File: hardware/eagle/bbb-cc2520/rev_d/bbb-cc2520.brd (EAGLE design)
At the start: 54.6 x 73.4 mm, 98 parts, among them J1 TC2030-IDC, J2 JUMPER-PTH-2-NO, P9/P8 BBB_HEADERS, U1 CC2520, U2 CC2520, U3 CAT24C256WI-GT3, U4 CC2591, U5 CD4051B-53B, U6 NRF51822QF, X1 NX2520SA, X2 NX2520SA, X3 16MHz

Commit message: committing changes to gap
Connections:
- removed net A0: U6.45
- removed net A1: U6.46
- removed net CC0_GPIO0: U1.10
- removed net CC0_GPIO5: U1.4
- removed net P03: U6.7
- removed net P12: U6.18
- removed net P24: U6.43
- removed net P25: U6.44
- removed net PROG_RX: U6.47
- removed net PROG_TX: U6.48
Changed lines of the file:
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@@
 <wire x1="13.462" y1="46.482" x2="12.192" y2="45.212" width="0.2032" layer="1"/>
-</signal>
-<signal name="CC0_GPIO5">
-<contactref element="U1" pad="4"/>
-</signal>
-<signal name="CC0_GPIO0">
-<contactref element="U1" pad="10"/>
 </signal>
 <signal name="VCC">
@@
 <wire x1="26.19593125" y1="56.093" x2="25.908" y2="55.80506875" width="0.2032" layer="1"/>
 <wire x1="25.908" y1="55.80506875" x2="24.892" y2="55.80506875" width="0.2032" layer="1"/>
-<contactref element="R15" pad="2"/>
-<contactref element="R16" pad="2"/>
-<via x="23.876" y="40.132" extent="1-16" drill="0.4064"/>
-<contactref element="R14" pad="2"/>
 <wire x1="13.02893125" y1="66.04" x2="11.35506875" y2="66.04" width="0.4064" layer="1"/>
 <wire x1="11.35506875" y1="64.135" x2="11.35506875" y2="66.04" width="0.4064" layer="1"/>
@@
 <via x="24.003" y="55.626" extent="1-16" drill="0.4064"/>
 <wire x1="7.884" y1="68.448" x2="7.874" y2="68.65493125" width="0.254" layer="1"/>
+<wire x1="32.58693125" y1="19.05" x2="32.3215" y2="18.78456875" width="0.2032" layer="1"/>
+<wire x1="32.3215" y1="18.78456875" x2="32.3215" y2="17.78" width="0.2032" layer="1"/>
+<wire x1="11.35506875" y1="66.04" x2="11.35506875" y2="68.20893125" width="0.4064" layer="1"/>
+<wire x1="11.35506875" y1="68.20893125" x2="11.116" y2="68.448" width="0.4064" layer="1"/>
+<wire x1="19.812" y1="40.894" x2="19.893" y2="40.813" width="0.2032" layer="1"/>
+<wire x1="19.893" y1="40.813" x2="19.893" y2="39.867" width="0.2032" layer="1"/>
+<contactref element="R15" pad="2"/>
+<contactref element="R16" pad="2"/>
+<contactref element="R14" pad="2"/>
+<via x="23.876" y="40.132" extent="1-16" drill="0.4064"/>
 <wire x1="24.05506875" y1="37.846" x2="24.05506875" y2="38.42893125" width="0.2032" layer="1"/>
 <wire x1="24.05506875" y1="38.42893125" x2="23.368" y2="39.116" width="0.2032" layer="1"/>
 <wire x1="23.368" y1="39.116" x2="22.78506875" y2="39.116" width="0.2032" layer="1"/>
 <wire x1="22.78506875" y1="41.148" x2="23.368" y2="41.148" width="0.2032" layer="1"/>
-<wire x1="32.58693125" y1="19.05" x2="32.3215" y2="18.78456875" width="0.2032" layer="1"/>
-<wire x1="32.3215" y1="18.78456875" x2="32.3215" y2="17.78" width="0.2032" layer="1"/>
-<wire x1="11.35506875" y1="66.04" x2="11.35506875" y2="68.20893125" width="0.4064" layer="1"/>
-<wire x1="11.35506875" y1="68.20893125" x2="11.116" y2="68.448" width="0.4064" layer="1"/>
 <wire x1="23.368" y1="41.148" x2="23.876" y2="40.64" width="0.2032" layer="1"/>
 <wire x1="23.876" y1="40.64" x2="23.876" y2="40.132" width="0.2032" layer="1"/>
 <wire x1="23.368" y1="39.116" x2="23.876" y2="39.624" width="0.2032" layer="1"/>
 <wire x1="23.876" y1="39.624" x2="23.876" y2="40.132" width="0.2032" layer="1"/>
-<wire x1="19.812" y1="40.894" x2="19.893" y2="40.813" width="0.2032" layer="1"/>
-<wire x1="19.893" y1="40.813" x2="19.893" y2="39.867" width="0.2032" layer="1"/>
 </signal>
 <signal name="LED2">
@@
 <wire x1="46.91506875" y1="67.38493125" x2="46.736" y2="67.38493125" width="0.4064" layer="1"/>
 </signal>
-<signal name="P12">
-<contactref element="U6" pad="18"/>
-</signal>
-<signal name="PROG_RX">
-<contactref element="U6" pad="47"/>
-</signal>
-<signal name="PROG_TX">
-<contactref element="U6" pad="48"/>
-</signal>
-<signal name="P25">
-<contactref element="U6" pad="44"/>
-</signal>
-<signal name="P24">
-<contactref element="U6" pad="43"/>
-</signal>
-<signal name="A1">
-<contactref element="U6" pad="46"/>
-</signal>
-<signal name="A0">
-<contactref element="U6" pad="45"/>
-</signal>
 <signal name="BIRQ">
 <contactref element="P9/P8" pad="P9_16"/>
@@
 <wire x1="22.457" y1="56.493" x2="20.828" y2="54.864" width="0.2032" layer="1"/>
 </signal>
-<signal name="P03">
-<contactref element="U6" pad="7"/>
-</signal>
 <signal name="SPI0_CS0_SEL0">

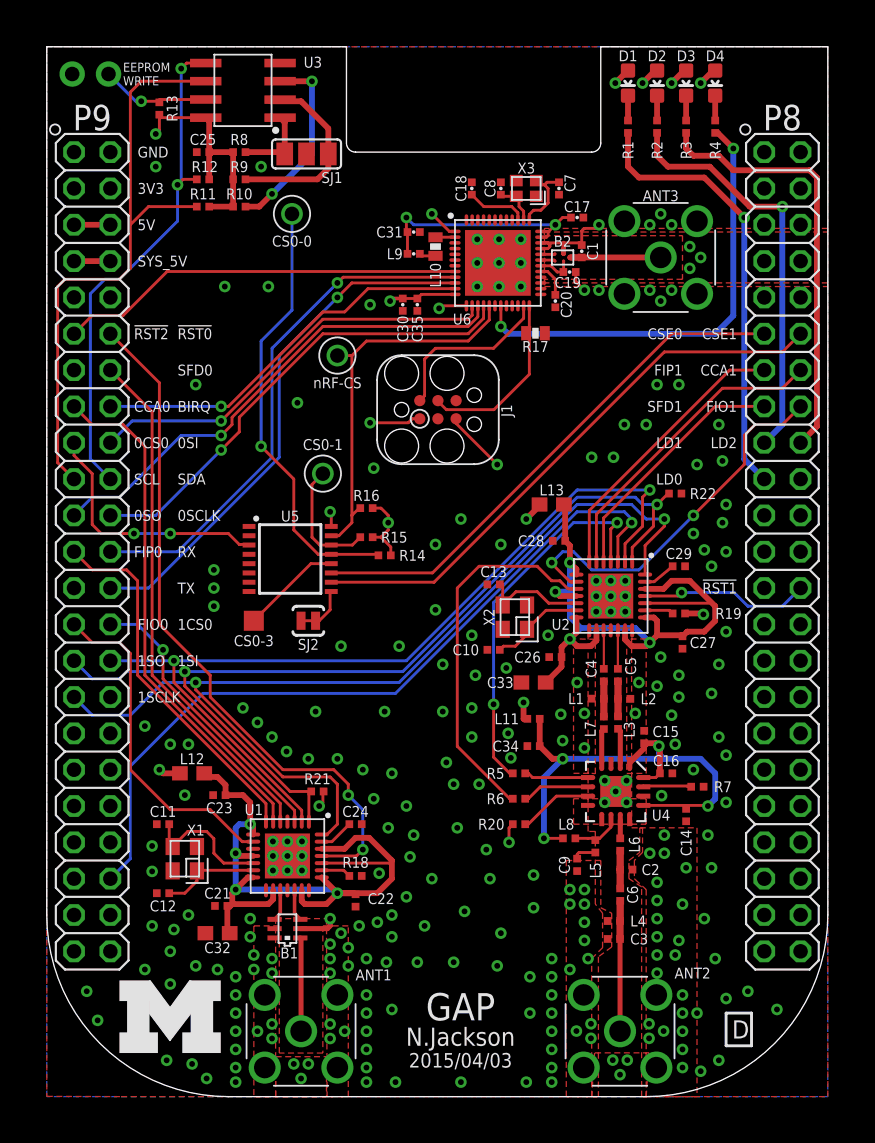
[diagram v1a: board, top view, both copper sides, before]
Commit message: mouse bites
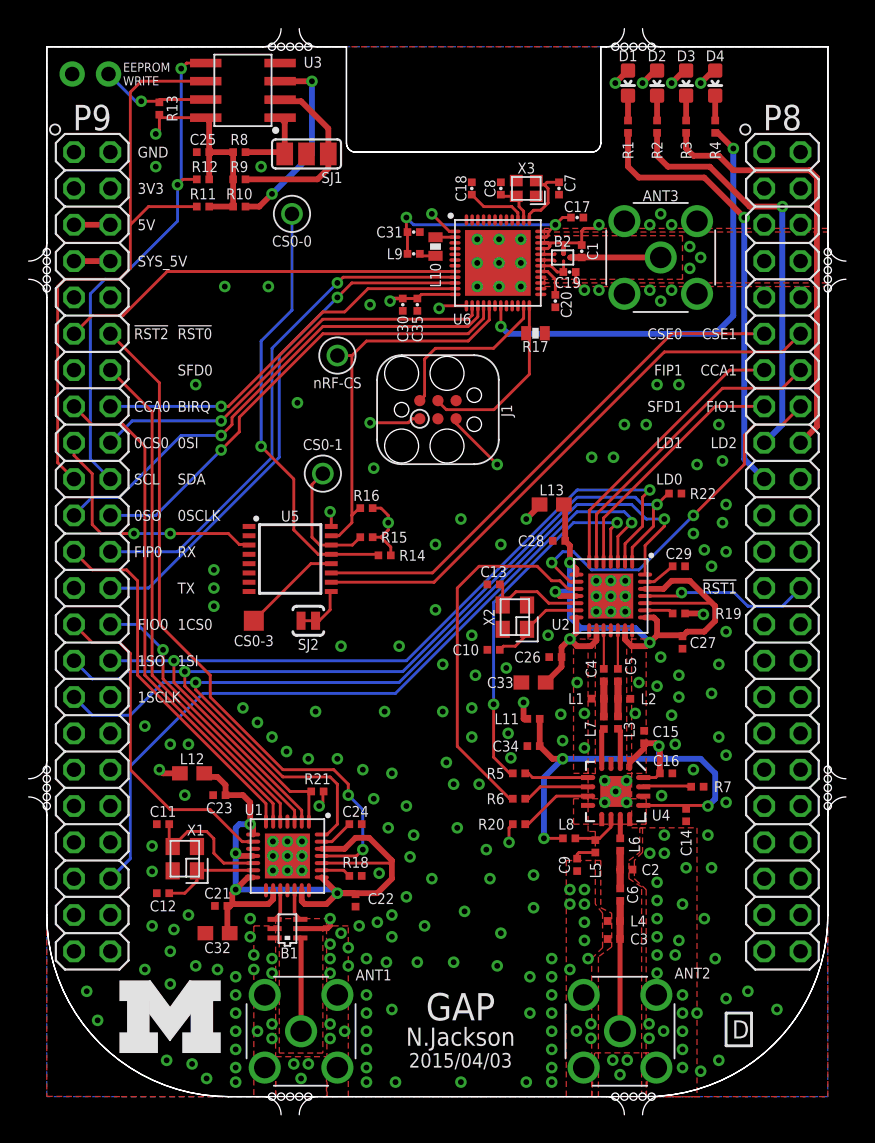
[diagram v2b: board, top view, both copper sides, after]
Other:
- board size 54.6 x 73.4 mm -> 57.2 x 75.9 mm
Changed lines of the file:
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@@
 <setting verticaltext="up"/>
 </settings>
-<grid distance="10" unitdist="mil" unit="mil" style="lines" multiple="1" display="yes" altdistance="5" altunitdist="mil" altunit="mil"/>
+<grid distance="50" unitdist="mil" unit="mil" style="lines" multiple="1" display="yes" altdistance="5" altunitdist="mil" altunit="mil"/>
 <layers>
 <layer number="1" name="Top" color="4" fill="1" visible="yes" active="yes"/>
@@
 <layer number="20" name="Dimension" color="15" fill="1" visible="yes" active="yes"/>
 <layer number="21" name="tPlace" color="7" fill="1" visible="yes" active="yes"/>
-<layer number="22" name="bPlace" color="7" fill="1" visible="yes" active="yes"/>
+<layer number="22" name="bPlace" color="7" fill="1" visible="no" active="yes"/>
 <layer number="23" name="tOrigins" color="15" fill="1" visible="yes" active="yes"/>
-<layer number="24" name="bOrigins" color="15" fill="1" visible="yes" active="yes"/>
+<layer number="24" name="bOrigins" color="15" fill="1" visible="no" active="yes"/>
 <layer number="25" name="tNames" color="7" fill="1" visible="yes" active="yes"/>
-<layer number="26" name="bNames" color="7" fill="1" visible="yes" active="yes"/>
+<layer number="26" name="bNames" color="7" fill="1" visible="no" active="yes"/>
 <layer number="27" name="tValues" color="7" fill="1" visible="no" active="yes"/>
 <layer number="28" name="bValues" color="7" fill="1" visible="no" active="yes"/>
@@
 <layer number="43" name="vRestrict" color="2" fill="10" visible="no" active="yes"/>
 <layer number="44" name="Drills" color="7" fill="1" visible="no" active="yes"/>
-<layer number="45" name="Holes" color="7" fill="1" visible="no" active="yes"/>
-<layer number="46" name="Milling" color="3" fill="1" visible="no" active="yes"/>
+<layer number="45" name="Holes" color="7" fill="1" visible="yes" active="yes"/>
+<layer number="46" name="Milling" color="3" fill="1" visible="yes" active="yes"/>
 <layer number="47" name="Measures" color="7" fill="1" visible="no" active="yes"/>
 <layer number="48" name="Document" color="7" fill="1" visible="no" active="yes"/>
@@
 <board>
 <plain>
-<wire x1="0" y1="73.406" x2="0" y2="12.7" width="0" layer="20"/>
-<wire x1="0" y1="12.7" x2="12.7" y2="0" width="0" layer="20" curve="90"/>
-<wire x1="12.7" y1="0" x2="41.91" y2="0" width="0" layer="20"/>
-<wire x1="41.91" y1="0" x2="54.61" y2="12.7" width="0" layer="20" curve="90"/>
-<wire x1="54.61" y1="12.7" x2="54.61" y2="73.406" width="0" layer="20"/>
-<wire x1="54.61" y1="73.406" x2="38.735" y2="73.406" width="0" layer="20"/>
-<wire x1="38.735" y1="73.406" x2="38.735" y2="66.675" width="0" layer="20"/>
-<wire x1="38.735" y1="66.675" x2="38.1" y2="66.04" width="0" layer="20" curve="-90"/>
-<wire x1="38.1" y1="66.04" x2="21.59" y2="66.04" width="0" layer="20"/>
-<wire x1="21.59" y1="66.04" x2="20.955" y2="66.675" width="0" layer="20" curve="-90"/>
-<wire x1="20.955" y1="66.675" x2="20.955" y2="73.406" width="0" layer="20"/>
+<wire x1="0" y1="73.406" x2="0" y2="12.7" width="0" layer="46"/>
+<wire x1="0" y1="12.7" x2="12.7" y2="0" width="0" layer="46" curve="90"/>
+<wire x1="12.7" y1="0" x2="41.91" y2="0" width="0" layer="46"/>
+<wire x1="41.91" y1="0" x2="54.61" y2="12.7" width="0" layer="46" curve="90"/>
+<wire x1="54.61" y1="12.7" x2="54.61" y2="73.406" width="0" layer="46"/>
+<wire x1="54.61" y1="73.406" x2="38.735" y2="73.406" width="0" layer="46"/>
+<wire x1="38.735" y1="73.406" x2="38.735" y2="66.675" width="0" layer="46"/>
+<wire x1="38.735" y1="66.675" x2="38.1" y2="66.04" width="0" layer="46" curve="-90"/>
+<wire x1="38.1" y1="66.04" x2="21.59" y2="66.04" width="0" layer="46"/>
+<wire x1="21.59" y1="66.04" x2="20.955" y2="66.675" width="0" layer="46" curve="-90"/>
+<wire x1="20.955" y1="66.675" x2="20.955" y2="73.406" width="0" layer="46"/>
 <text x="6.35" y="4.191" size="0.762" layer="51" font="vector" ratio="10" rot="R90" align="top-center">SDA</text>
 <text x="6.35" y="6.731" size="0.762" layer="51" font="vector" ratio="10" rot="R90" align="top-center">SCL</text>
@@
 <text x="48.514" y="4.064" size="1.27" layer="21" font="vector" ratio="14" align="bottom-center">D</text>
 <text x="9.144" y="48.26" size="0.762" layer="25" font="vector" ratio="12" align="center-left">BIRQ</text>
-<wire x1="20.955" y1="73.406" x2="0" y2="73.406" width="0" layer="20"/>
+<wire x1="20.955" y1="73.406" x2="0" y2="73.406" width="0" layer="46"/>
 <text x="5.334" y="71.501" size="0.635" layer="21" font="vector" ratio="12" align="center-left">EEPROM
 WRITE</text>
@@
 <text x="9.144" y="30.48" size="0.762" layer="25" font="vector" ratio="12" align="center-left">1SI</text>
 <text x="6.35" y="27.94" size="0.762" layer="25" font="vector" ratio="12" align="center-left">1SCLK</text>
+<wire x1="0" y1="73.406" x2="0" y2="59.69" width="0" layer="20"/>
+<wire x1="0" y1="55.88" x2="0" y2="23.495" width="0" layer="20"/>
+<wire x1="0" y1="19.685" x2="0" y2="12.7" width="0" layer="20"/>
+<wire x1="0" y1="12.7" x2="12.7" y2="0" width="0" layer="20" curve="90"/>
+<wire x1="12.7" y1="0" x2="15.113" y2="0" width="0" layer="20"/>
+<wire x1="18.923" y1="0" x2="39.116" y2="0" width="0" layer="20"/>
+<wire x1="42.926" y1="0.040640625" x2="54.61" y2="12.7" width="0" layer="20" curve="85.5"/>
+<wire x1="54.61" y1="12.7" x2="54.61" y2="19.685" width="0" layer="20"/>
+<wire x1="54.61" y1="23.495" x2="54.61" y2="55.88" width="0" layer="20"/>
+<wire x1="54.61" y1="59.69" x2="54.61" y2="73.406" width="0" layer="20"/>
+<wire x1="54.61" y1="73.406" x2="42.926" y2="73.406" width="0" layer="20"/>
+<wire x1="39.116" y1="73.406" x2="38.735" y2="73.406" width="0" layer="20"/>
+<wire x1="38.735" y1="73.406" x2="38.735" y2="66.675" width="0" layer="20"/>
+<wire x1="38.735" y1="66.675" x2="38.1" y2="66.04" width="0" layer="20" curve="-90"/>
+<wire x1="38.1" y1="66.04" x2="21.59" y2="66.04" width="0" layer="20"/>
+<wire x1="21.59" y1="66.04" x2="20.955" y2="66.675" width="0" layer="20" curve="-90"/>
+<wire x1="20.955" y1="66.675" x2="20.955" y2="73.406" width="0" layer="20"/>
+<wire x1="20.955" y1="73.406" x2="18.923" y2="73.406" width="0" layer="20"/>
+<wire x1="15.113" y1="73.406" x2="0" y2="73.406" width="0" layer="20"/>
+<wire x1="0" y1="23.495" x2="-1.27" y2="22.225" width="0" layer="20" curve="-90"/>
+<wire x1="-1.27" y1="20.955" x2="0" y2="19.685" width="0" layer="20" curve="-90"/>
+<hole x="0" y="21.59" drill="0.508"/>
+<hole x="0" y="22.225" drill="0.508"/>
+<hole x="0" y="22.86" drill="0.508"/>
+<hole x="0" y="20.955" drill="0.508"/>
+<hole x="0" y="20.32" drill="0.508"/>
+<wire x1="0" y1="59.69" x2="-1.27" y2="58.42" width="0" layer="20" curve="-90"/>
+<wire x1="-1.27" y1="57.15" x2="0" y2="55.88" width="0" layer="20" curve="-90"/>
+<hole x="0" y="57.785" drill="0.508"/>
+<hole x="0" y="58.42" drill="0.508"/>
+<hole x="0" y="59.055" drill="0.508"/>
+<hole x="0" y="57.15" drill="0.508"/>
+<hole x="0" y="56.515" drill="0.508"/>
+<hole x="54.61" y="57.785" drill="0.508"/>
+<hole x="54.61" y="57.15" drill="0.508"/>
+<hole x="54.61" y="56.515" drill="0.508"/>
+<hole x="54.61" y="58.42" drill="0.508"/>
+<hole x="54.61" y="59.055" drill="0.508"/>
+<wire x1="54.61" y1="59.69" x2="55.88" y2="58.42" width="0" layer="20" curve="90"/>
+<wire x1="55.88" y1="57.15" x2="54.61" y2="55.88" width="0" layer="20" curve="90"/>
+<wire x1="54.61" y1="23.495" x2="55.88" y2="22.225" width="0" layer="20" curve="90"/>
+<wire x1="55.88" y1="20.955" x2="54.61" y2="19.685" width="0" layer="20" curve="90"/>
+<hole x="54.61" y="21.59" drill="0.508"/>
+<hole x="54.61" y="22.225" drill="0.508"/>
+<hole x="54.61" y="22.86" drill="0.508"/>
+<hole x="54.61" y="20.955" drill="0.508"/>
+<hole x="54.61" y="20.32" drill="0.508"/>
+<wire x1="39.116" y1="73.406" x2="40.386" y2="74.676" width="0" layer="20" curve="90"/>
+<wire x1="41.656" y1="74.676" x2="42.926" y2="73.406" width="0" layer="20" curve="90"/>
+<hole x="41.021" y="73.406" drill="0.508"/>
+<hole x="41.656" y="73.406" drill="0.508"/>
+<hole x="42.291" y="73.406" drill="0.508"/>
+<hole x="40.386" y="73.406" drill="0.508"/>
+<hole x="39.751" y="73.406" drill="0.508"/>
+<wire x1="15.113" y1="73.406" x2="16.383" y2="74.676" width="0" layer="20" curve="90"/>
+<wire x1="17.653" y1="74.676" x2="18.923" y2="73.406" width="0" layer="20" curve="90"/>
+<hole x="17.018" y="73.406" drill="0.508"/>
+<hole x="17.653" y="73.406" drill="0.508"/>
+<hole x="18.288" y="73.406" drill="0.508"/>
+<hole x="16.383" y="73.406" drill="0.508"/>
+<hole x="15.748" y="73.406" drill="0.508"/>
+<wire x1="18.923" y1="0" x2="17.653" y2="-1.27" width="0" layer="20" curve="90"/>
+<wire x1="16.383" y1="-1.27" x2="15.113" y2="0" width="0" layer="20" curve="90"/>
+<hole x="17.018" y="0" drill="0.508"/>
+<hole x="16.383" y="0" drill="0.508"/>
+<hole x="15.748" y="0" drill="0.508"/>
+<hole x="17.653" y="0" drill="0.508"/>
+<hole x="18.288" y="0" drill="0.508"/>
+<wire x1="42.926" y1="0.040640625" x2="41.656" y2="-1.27" width="0" layer="20" curve="87"/>
+<wire x1="40.386" y1="-1.27" x2="39.116" y2="0" width="0" layer="20" curve="90"/>
+<hole x="41.021" y="0" drill="0.508"/>
+<hole x="40.386" y="0" drill="0.508"/>
+<hole x="39.751" y="0" drill="0.508"/>
+<hole x="41.656" y="0" drill="0.508"/>
+<hole x="42.291" y="0" drill="0.508"/>
 </plain>
 <attributes>
